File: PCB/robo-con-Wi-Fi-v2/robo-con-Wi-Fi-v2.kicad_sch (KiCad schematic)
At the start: 109 parts, among them J1 Conn_01x04, J2 SMA-J, J3 Conn_01x05, J4 Conn_01x01, J5 Conn_01x02, J6 Conn_01x01, J7 Conn_01x06, J8 Conn_01x01, J9 Conn_01x01, SW1 SW_Push, SW2 SW_Slide, U1 STM32H723VGTx, U10 MCP73831-2-OT, U11 LM66100DCK, U15 LM66100DCK, U18 USB_Type-C, U2 LBEE5HY2FY, U3 FT234XD, U4 MCP1727-1802xMF, U5 RKJXV122400R, U6 LD39200PU33R, U7 RKJXV122400R, U8 TMHU28, U9 TMHU28, Y2 XRCGB25M000FFS1AR0

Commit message: v2 配線
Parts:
- removed R1, R31: WA04X102, My_Library:WA04X102, symbol My_Library:WA04X102
- removed R28, R29: 10k, Resistor_SMD:R_0603_1608Metric_Pad0.98x0.95mm_HandSolder, symbol Device:R_Small
- removed R30, R47, R7: 1k, Resistor_SMD:R_0402_1005Metric_Pad0.72x0.64mm_HandSolder, symbol Device:R_Small
- added D15: W, Diode_SMD:D_0603_1608Metric_Pad1.05x0.95mm_HandSolder, symbol Device:LED_Small
- added D17: O, Diode_SMD:D_0603_1608Metric_Pad1.05x0.95mm_HandSolder, symbol Device:LED_Small
- added D18: R, Diode_SMD:D_0603_1608Metric_Pad1.05x0.95mm_HandSolder, symbol Device:LED_Small
- added R12, R13, R14, R15: 10k, Resistor_SMD:R_0402_1005Metric_Pad0.72x0.64mm_HandSolder, symbol Device:R_Small
- added R22, R34, R36: 1k, Resistor_SMD:R_0402_1005Metric_Pad0.72x0.64mm_HandSolder, symbol Device:R_Small
- F1: value box -> FHC16322ADTP
- SW2: value SW_Slide -> SS-12D00G3
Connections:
- net L1_BUTTON is gone; now on net R1_BUTTON: J7.2 (Pin_2)
- net L2_BUTTON is gone; now on net R2_BUTTON: J7.3 (Pin_3)
- net L3_BUTTON is gone; now on net R3_BUTTON: J7.4 (Pin_4)
- net L4_BUTTON is gone; now on net R4_BUTTON: J7.5 (Pin_5)
- net R5_BUTTON is gone; now on net L5_BUTTON: J3.2 (Pin_2)
- net R6_BUTTON is gone; now on net L6_BUTTON: J3.3 (Pin_3)
- net R7_BUTTON is gone; now on net L7_BUTTON: J3.4 (Pin_4)
- net +3.3V: now also D1.2 (A), D10.2 (A), D13.2 (A), D14.2 (A), D16.2 (A), D3.2 (A), D5.2 (A), D17.2 (A), D18.2 (A); no longer R11.1, R2.1, R32.1, R33.1, R35.1, R4.1, R6.1
- net +5V: now also R22.1
- net BT_ON: now also U1.87 (PD6)
- net GND: now also D15.1 (K), R12.2, R13.2, R14.2, R15.2
- net L0_LEVER: now also U1.1 (PE2)
- net L1_LEVER: now also U1.3 (PE4)
- net L2_LEVER: now also U1.2 (PE3)
- net L3_LEVER: now also U1.4 (PE5)
- net L4_LEVER: now also U1.5 (PE6)
- net LED0: now also R2.2, U1.89 (PB3(JTDO); no longer D1.1 (K)
- net LED1: now also R4.2, U1.90 (PB4(NJTRST)); no longer D3.1 (K)
- net LED2: now also R6.2, U1.91 (PB5); no longer D5.1 (K)
- net LED3: now also R11.2, U1.92 (PB6); no longer D10.1 (K)
- net LED4: now also R32.2, U1.93 (PB7); no longer D13.1 (K)
- net LEDUSB: now also U1.96 (PB9), R34.2
- net LEDWL: now also R33.2, U1.95 (PB8); no longer D14.1 (K)
- net LP_STICK: now also U1.30 (PA6)
- net LX_STICK: now also U1.29 (PA5), R13.1
- net LY_STICK: now also U1.28 (PA4), R12.1
- net LiPo_OBSERVE: now also U1.33 (PC5)
- net R0_LEVER: now also U1.61 (PD14)
- net R1_LEVER: now also U1.63 (PC6)
- net R2_LEVER: now also U1.62 (PD15)
- net R3_LEVER: now also U1.60 (PD13)
- net R4_LEVER: now also U1.57 (PD10)
- net RP_STICK: now also U1.47 (PB11)
- net RX_STICK: now also U1.34 (PB0), R14.1
- net RY_STICK: now also U1.35 (PB1), R15.1
- net SDMMC1_CLK: now also R44.7; no longer R44.6
- net SDMMC1_CMD: now also R44.8; no longer R44.5
- net SDMMC1_D2: now also R44.5
- net SDMMC1_D3: now also R44.6; no longer R44.7
- net WL_ON: now also U1.86 (PD5)
- net R1_BUTTON: now reaches U1.51 (PB12)
- net R2_BUTTON: now reaches U1.52 (PB13)
- net R3_BUTTON: now reaches U1.53 (PB14)
- net R4_BUTTON: now reaches U1.54 (PB15)
- net L5_BUTTON: now reaches U1.7 (PC13)
- net L6_BUTTON: now reaches U1.8 (PC14)
- net L7_BUTTON: now reaches U1.9 (PC15)
- net LEDLiPo_GOOD: now reaches U1.97 (PE0)
- net LEDLiPo_GOOD: now also R35.2
- net LEDLiPo_BAD: now reaches U1.98 (PE1)
- net LEDLiPo_BAD: now also R36.2
- net LEDLiPo: no longer names the net of D16.1 (K)
- net LEDLiPo: now also R35.1
- new net: D13.1 (K), R32.1
- new net: D1.1 (K), R2.1
- new net: D3.1 (K), R4.1
- new net: D17.1 (K), R34.1
- new net: D18.1 (K), R36.1
- new net: D15.2 (A), R22.2
- new net: D5.1 (K), R6.1
- new net: D10.1 (K), R11.1
- new net: D14.1 (K), R33.1
- no-connect marks 35 -> 34
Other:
- moved on the sheet: D1, D10, D11, D13, D14, D16, D3, D5, J3, J7, R11, R2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

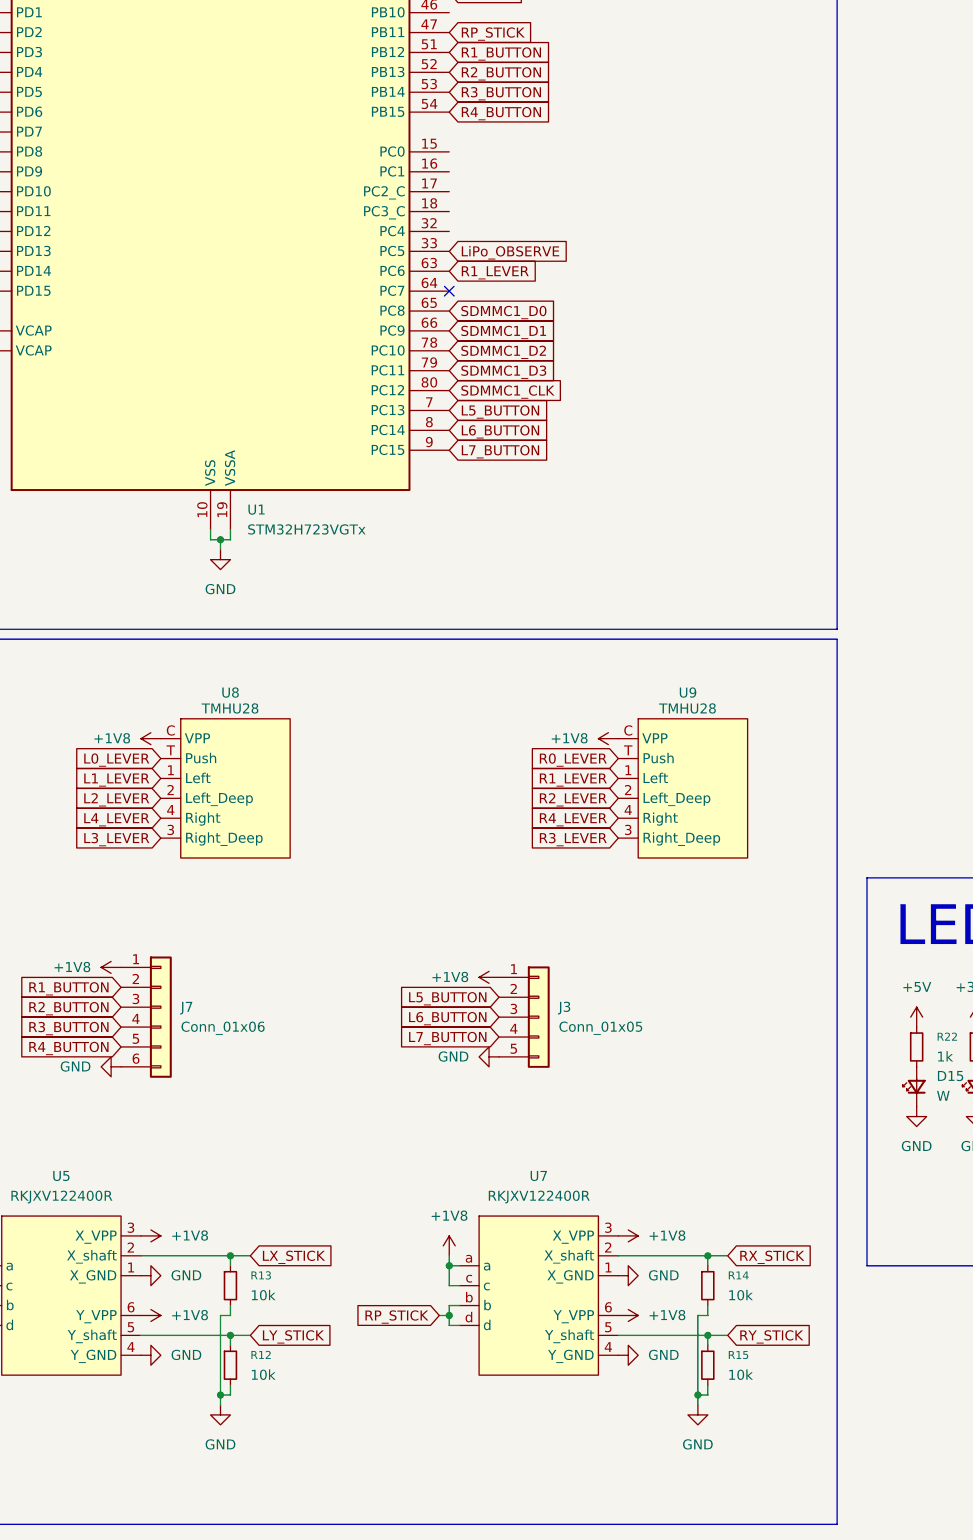
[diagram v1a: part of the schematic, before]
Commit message: PCB
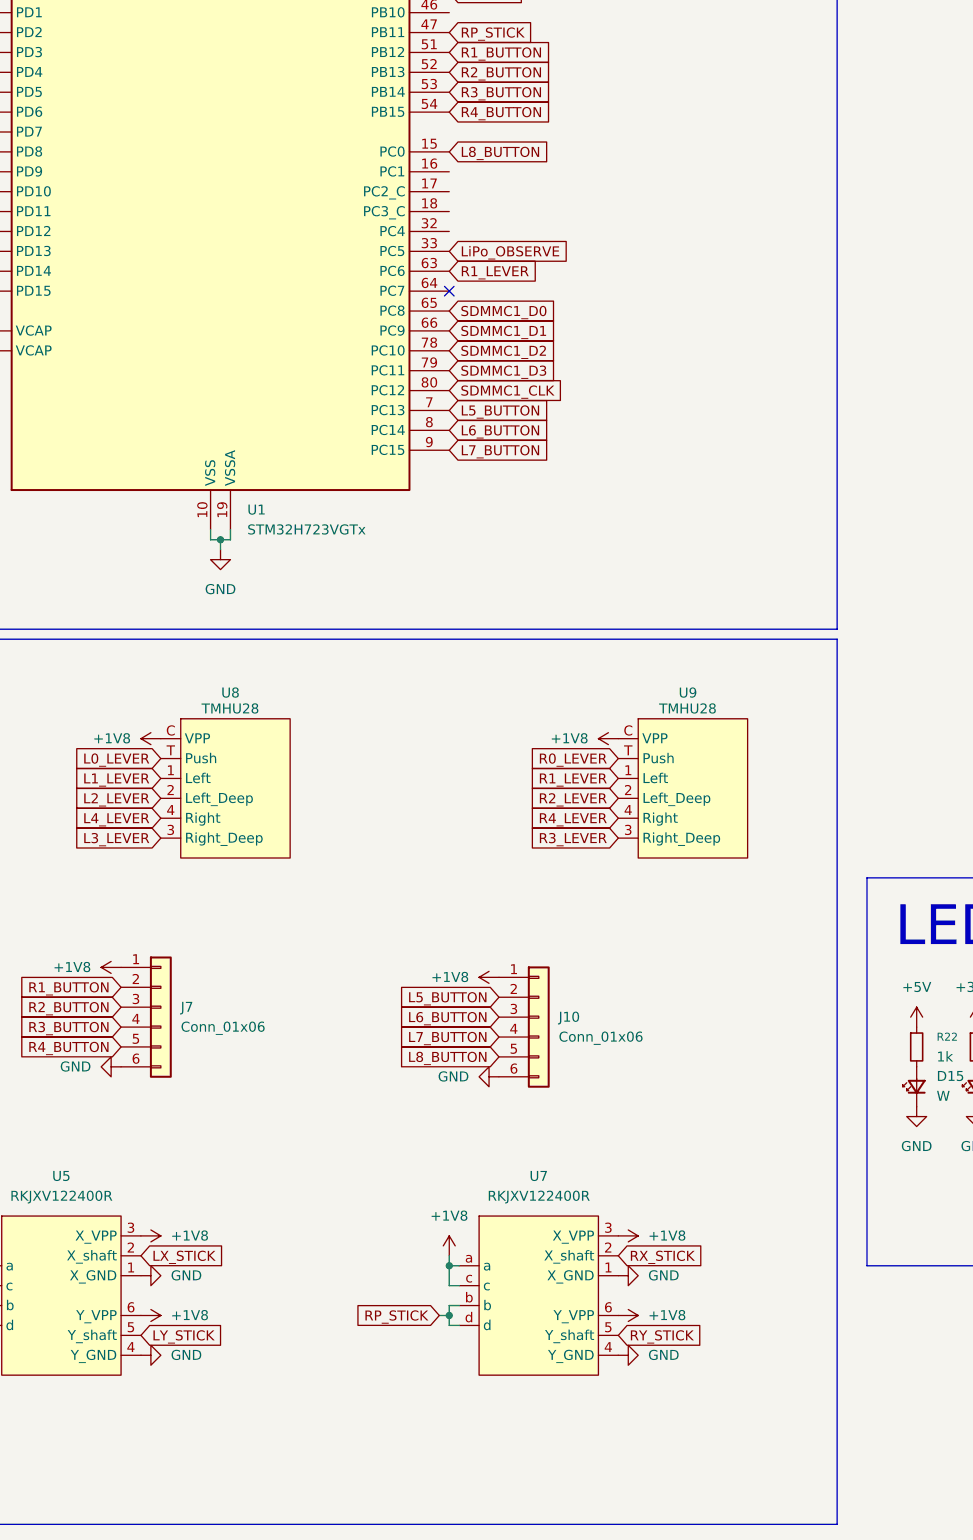
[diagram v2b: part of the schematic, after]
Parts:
- removed J3: Conn_01x05, Connector_JST:JST_ZH_B5B-ZR_1x05_P1.50mm_Vertical, symbol Connector_Generic:Conn_01x05
- removed R12, R13, R14, R15: 10k, Resistor_SMD:R_0402_1005Metric_Pad0.72x0.64mm_HandSolder, symbol Device:R_Small
- added J10: Conn_01x06, Connector_JST:JST_ZH_B6B-ZR_1x06_P1.50mm_Vertical, symbol Connector_Generic:Conn_01x06
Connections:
- net +1V8: now also J10.1 (Pin_1)
- net GND: now also J10.6 (Pin_6)
- net L5_BUTTON: now also J10.2 (Pin_2)
- net L6_BUTTON: now also J10.3 (Pin_3)
- net L7_BUTTON: now also J10.4 (Pin_4)
- net L8_BUTTON: now reaches U1.15 (PC0)
- net L8_BUTTON: now also J10.5 (Pin_5)
